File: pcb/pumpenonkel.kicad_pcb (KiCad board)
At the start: 2 copper layers, 113.1 x 135.9 mm, 54 parts, among them J1 Conn_01x03_Pin, J10 CHANNEL, J11 CHANNEL, J12 CHANNEL, J13 Screw_Terminal_01x02, J14 Screw_Terminal_01x02, J15 CHANNEL, J16 Conn_01x03_Pin, J17 Barrel_Jack, J2 Conn_01x03_Pin, J3 Conn_01x03_Pin, J4 Conn_01x03_Pin, J5 Conn_01x03_Pin, J6 Conn_01x03_Pin, J7 Conn_01x08_Pin, J8 CHANNEL, J9 CHANNEL, K1 SANYOU_SRD_Form_C, K2 SANYOU_SRD_Form_C, K3 SANYOU_SRD_Form_C, K4 SANYOU_SRD_Form_C, K5 SANYOU_SRD_Form_C, K6 SANYOU_SRD_Form_C, Q1 BC337, Q2 BC337, Q3 BC337, Q4 BC337, Q5 BC337, Q6 BC337

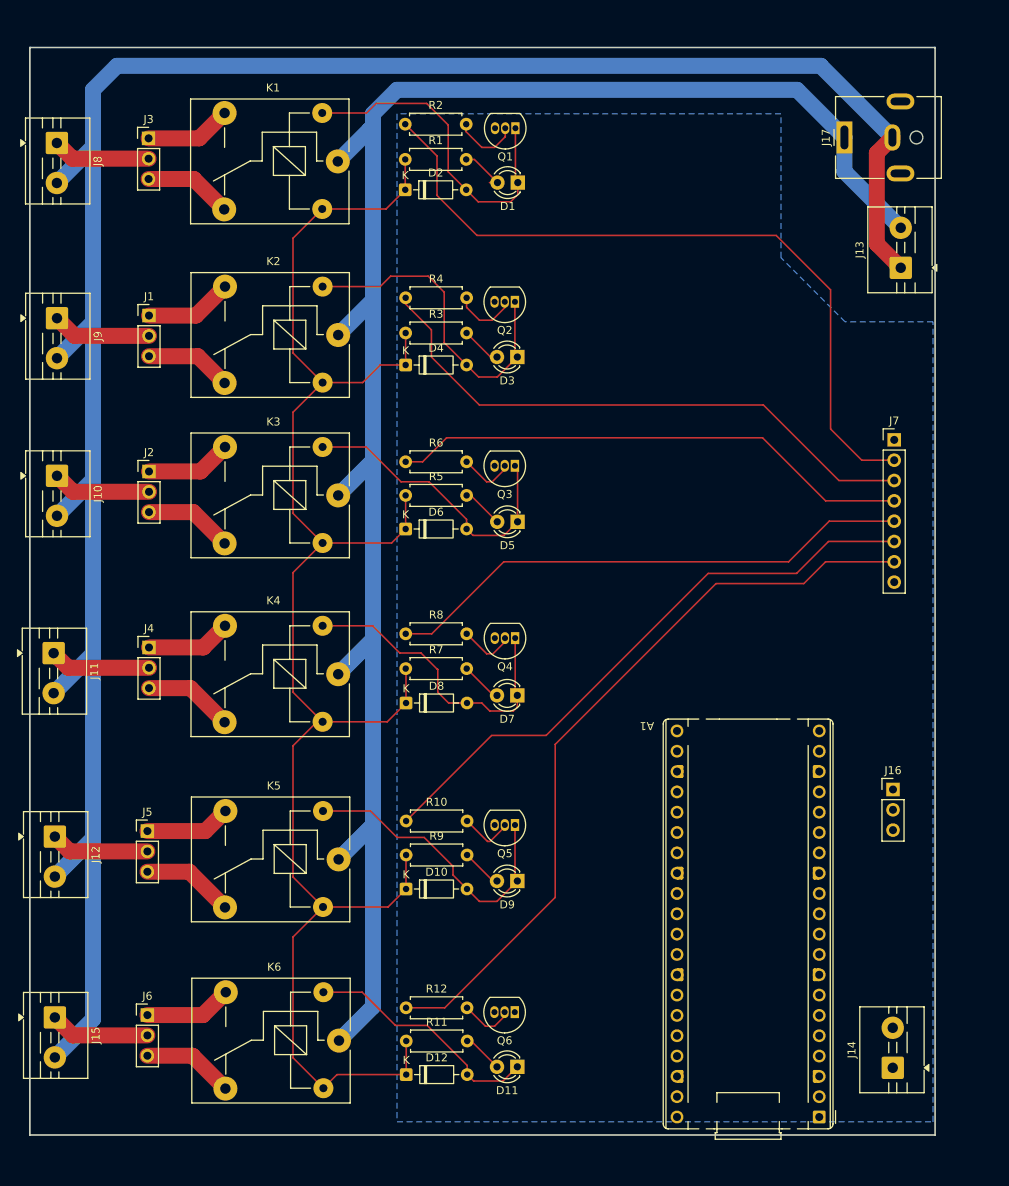
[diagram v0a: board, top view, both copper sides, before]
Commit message: finalilise pcb
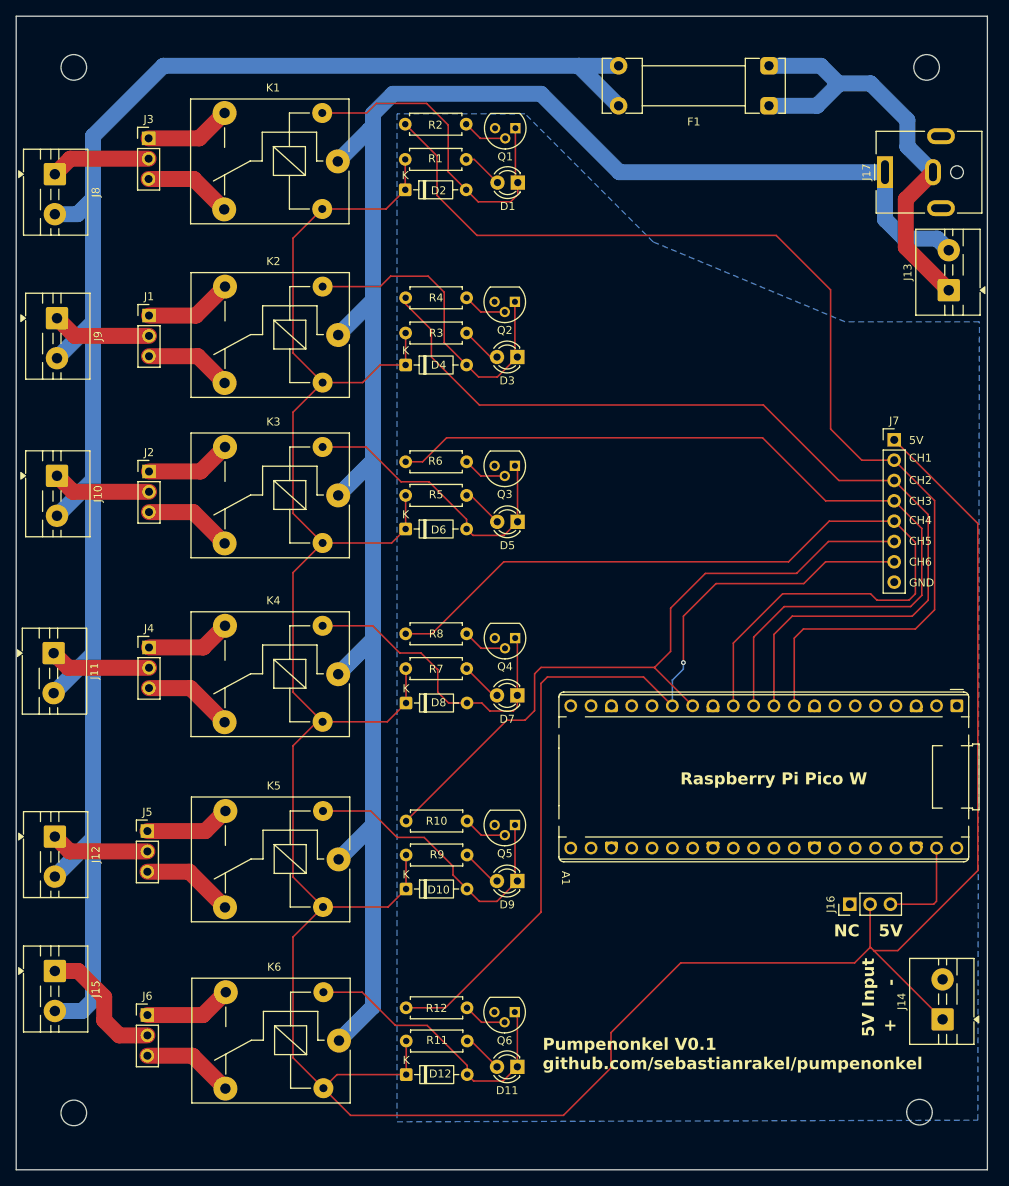
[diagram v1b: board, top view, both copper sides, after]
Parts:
- added F1: Fuse, Fuse:Fuseholder_Clip-5x20mm_Littelfuse_111_Lateral_P18.80x5.00mm_D1.17mm_Horizontal, F.Cu at (116.5, 35.0)
- Q1, Q2, Q3, Q4, Q5, Q6: footprint Package_TO_SOT_THT:TO-92_Inline -> Package_TO_SOT_THT:TO-92
- moved A1 54.2 mm to (140.0, 110.0), turned to -90 degrees
- moved J16 15.3 mm to (126.6, 134.8), turned to 90 degrees
- moved J14 8.69 mm to (138.2, 149.2)
- moved J17 6.67 mm to (131.0, 43.3)
- moved J13 6.62 mm to (139.0, 58.0)
- moved J15 5.80 mm to (27.2, 143.2)
- moved J8 3.91 mm to (27.2, 43.5)
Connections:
- J13 pad 1: VAC -> Net-(J13-Pin_1)
- J17 pad 2: VAC -> Net-(J13-Pin_1)
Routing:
- net VCC: track 218.0 -> 392.5 mm
- net VAC: track 279.0 -> 221.7 mm
- net Net-(J13-Pin_1): track 0.00 -> 56.2 mm
- net CH1: track 91.6 -> 139.9 mm
- net CH2: track 73.0 -> 119.7 mm
- net CH3: track 65.6 -> 110.6 mm
- net CH4: track 66.9 -> 110.9 mm
- net CH6: track 95.3 -> 109.6 mm, vias 0 -> 1
- net CH5: track 75.5 -> 88.1 mm
- net Net-(A1-VSYS): track 0.00 -> 12.6 mm
- net COM: track 225.0 -> 232.7 mm
- net Net-(D11-K): track 30.2 -> 37.2 mm
- net Net-(J15-Pin_1): track 12.5 -> 16.6 mm
- net Net-(Q1-B): track 8.26 -> 5.61 mm
- net Net-(Q2-B): track 8.01 -> 5.50 mm
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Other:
- board size 113.1 x 135.9 mm -> 121.4 x 144.2 mm
- board text added: "+"
- board text added: "-"
- board text added: "5V"
- board text added: "5V Input"
- board text added: "CH1"
- board text added: "CH2"
- board text added: "CH3"
- board text added: "CH4"
- board text added: "CH5"
- board text added: "CH6"
- board text added: "GND"
- board text added: "NC"
- board text added: "Pumpenonkel V0.1 github.com/sebastianrakel/pumpenonkel"
- board text added: "Raspberry Pi Pico W"
